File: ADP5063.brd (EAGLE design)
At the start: 33 x 14.9 mm, 23 parts, among them X1 PIIKKIRIMA-5, X2 PIIKKIRIMA-5, X3 PIIKKIRIMA-5, X4 PIIKKIRIMA-5, X5 629105136821

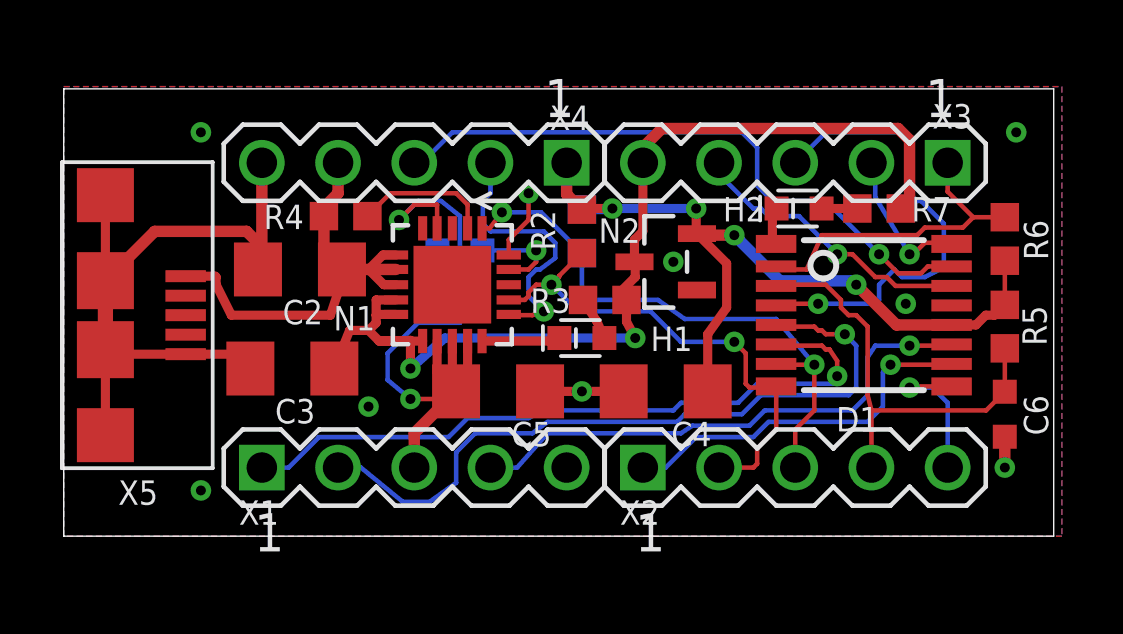
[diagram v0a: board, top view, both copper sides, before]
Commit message: Added avatar
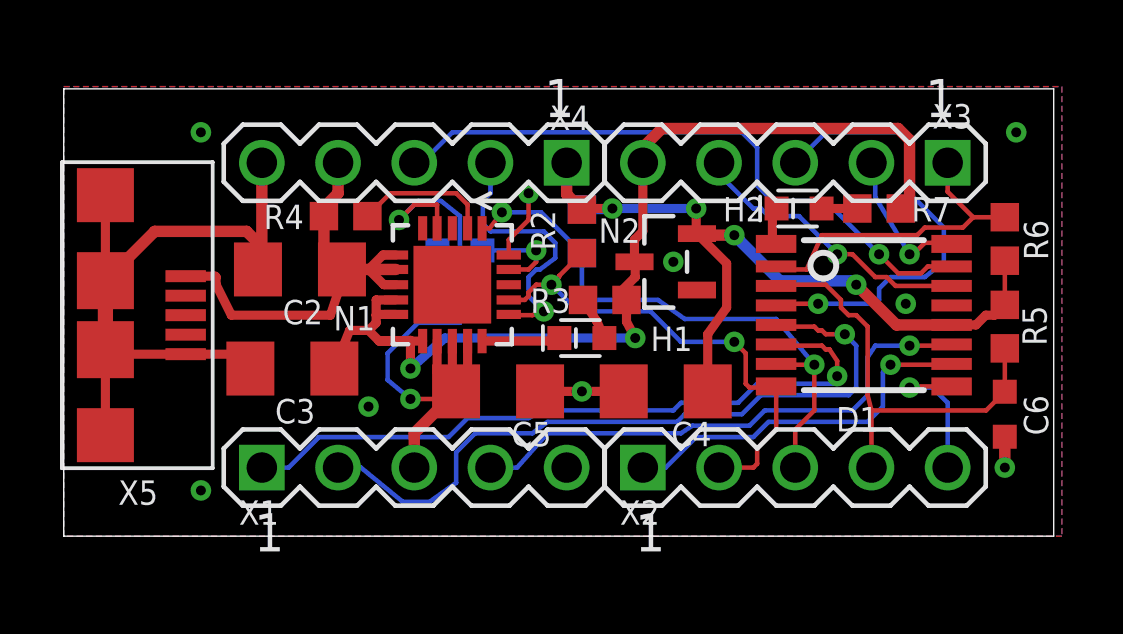
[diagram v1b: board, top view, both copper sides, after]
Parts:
- added U$1: (no value), dafug:DAFUG-.SM
